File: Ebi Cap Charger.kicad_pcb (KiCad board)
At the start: 2 copper layers, 45 x 100 mm, 31 parts, among them Q1 FET, Q2 FET, U1 LT3751, U2 DA2034-AL, U3 DA2034-AL, U4 DA2034-AL

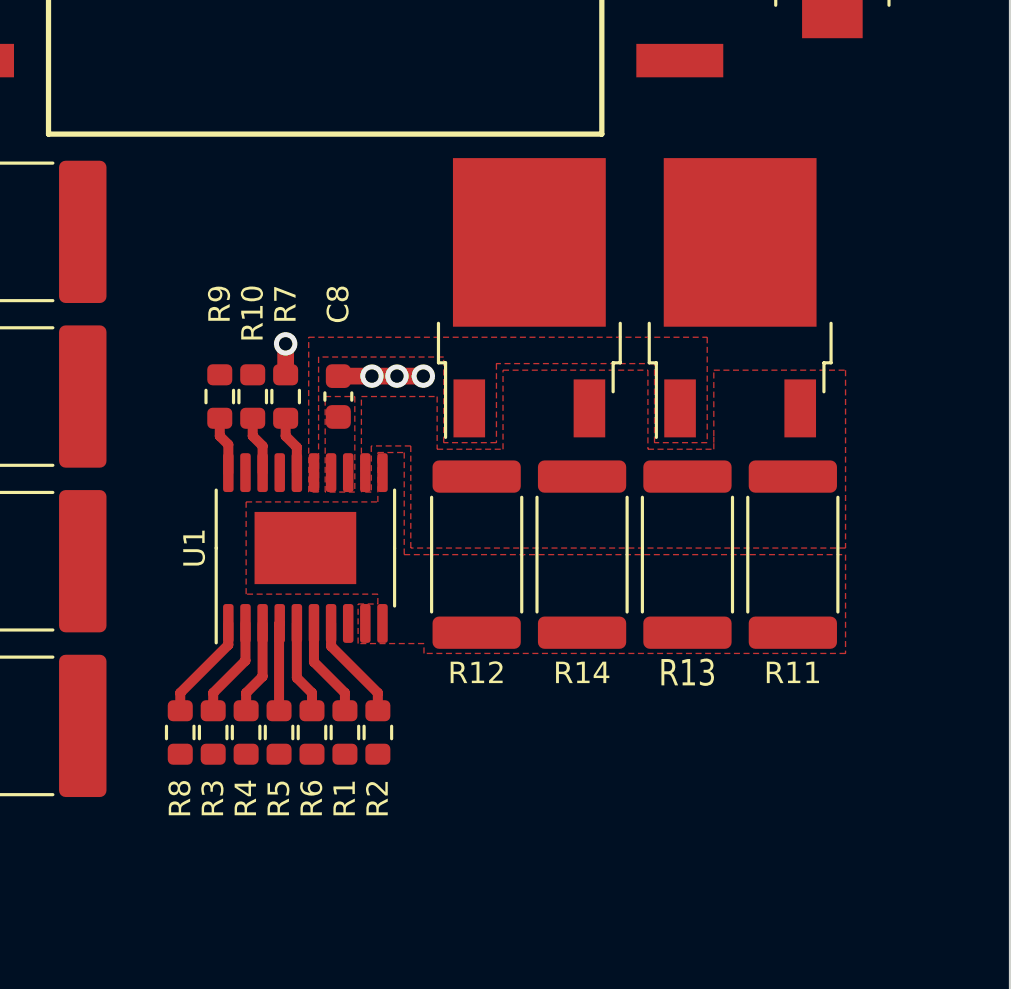
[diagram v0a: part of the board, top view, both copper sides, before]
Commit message: Updated PCB
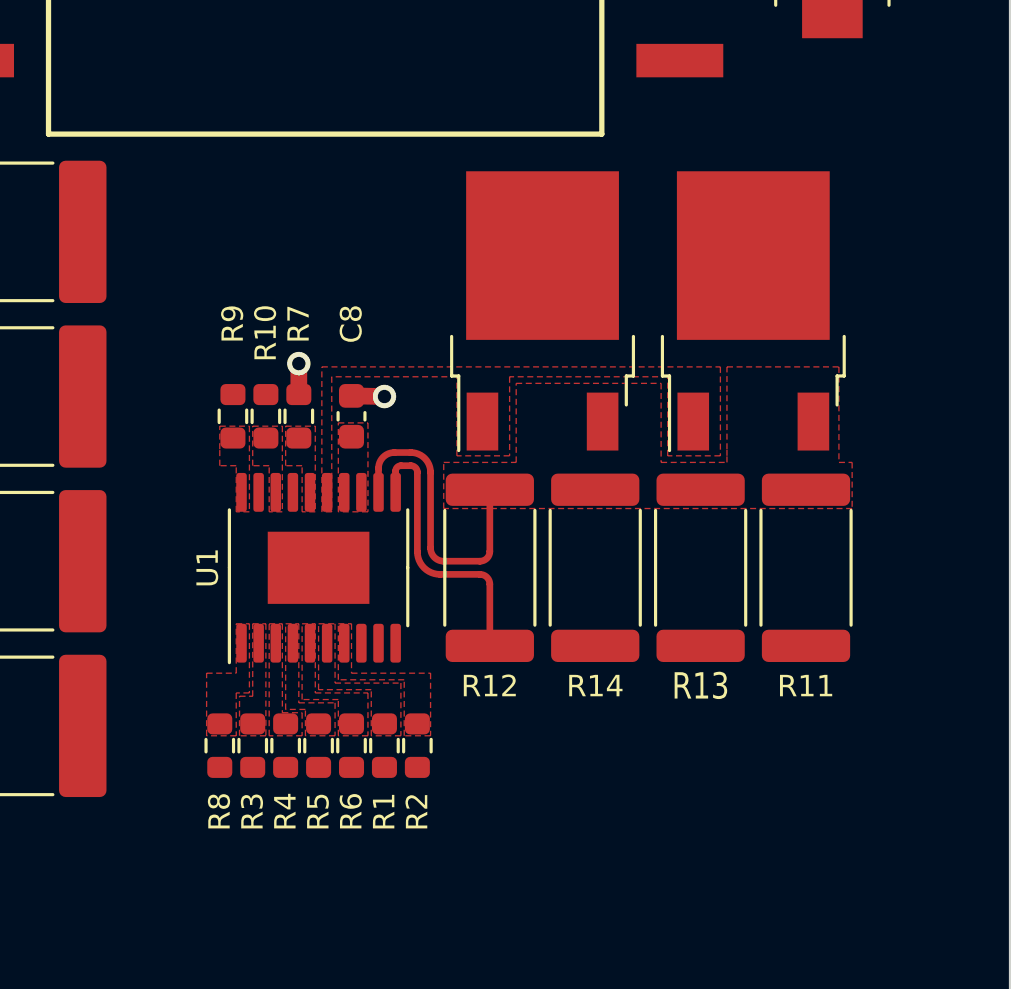
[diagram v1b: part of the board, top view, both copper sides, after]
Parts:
- moved R1 1.58 mm to (168.2, 195.5)
- moved R2 1.58 mm to (169.5, 195.5)
- moved R3 1.58 mm to (163.2, 195.5)
- moved R4 1.58 mm to (164.5, 195.5)
- moved R5 1.58 mm to (165.8, 195.5)
- moved R6 1.58 mm to (167.0, 195.5)
- moved R8 1.58 mm to (162.0, 195.5)
- moved C8 0.90 mm to (167.0, 183.0)
- moved R10 0.90 mm to (163.8, 183.0)
- moved R7 0.90 mm to (165.0, 183.0)
- moved R9 0.90 mm to (162.5, 183.0)
- moved U1 0.90 mm to (165.8, 188.8)
- moved Q1 0.71 mm to (174.2, 179.0)
- moved Q2 0.71 mm to (182.2, 179.0)
- moved R11 0.71 mm to (184.2, 188.8)
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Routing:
- net Net-(Q1-Pad3): track 0.00 -> 11.5 mm
- net GND: track 4.40 -> 13.1 mm, vias 4 -> 2
- net Net-(R8-Pad1): track 4.07 -> 0.00 mm
- net Net-(R2-Pad2): track 4.05 -> 0.00 mm
- net Net-(R3-Pad2): track 3.82 -> 0.00 mm
- net Net-(R1-Pad2): track 3.80 -> 0.00 mm
- net Net-(R4-Pad2): track 3.57 -> 0.00 mm
- net Net-(R6-Pad2): track 3.55 -> 0.00 mm
- net Net-(R5-Pad2): track 3.32 -> 0.00 mm
- net Net-(R7-Pad1): track 2.24 -> 0.00 mm
- net Net-(R10-Pad1): track 2.22 -> 0.00 mm
- net Net-(R9-Pad1): track 2.20 -> 0.00 mm
- added copper zone on F.Cu, net Net-(R1-Pad2)
- added copper zone on F.Cu, net Net-(R10-Pad1)
- added copper zone on F.Cu, net Net-(R2-Pad2)
- added copper zone on F.Cu, net Net-(R3-Pad2)
- added copper zone on F.Cu, net Net-(R4-Pad2)
- added copper zone on F.Cu, net Net-(R5-Pad2)
- added copper zone on F.Cu, net Net-(R6-Pad2)
- added copper zone on F.Cu, net Net-(R7-Pad1)
- added copper zone on F.Cu, net Net-(R8-Pad1)
- added copper zone on F.Cu, net Net-(R9-Pad1)
- removed copper zone on F.Cu, net GND

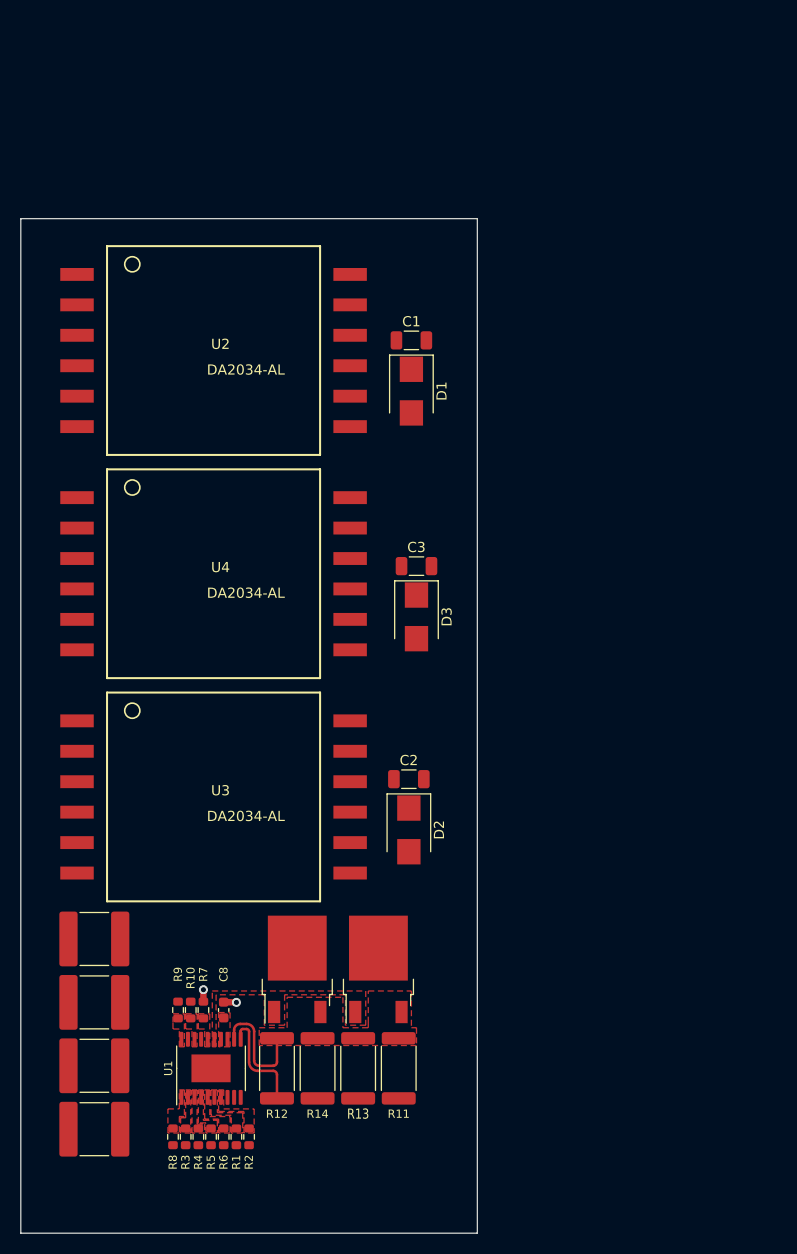
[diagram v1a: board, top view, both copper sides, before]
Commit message: Updated PCB
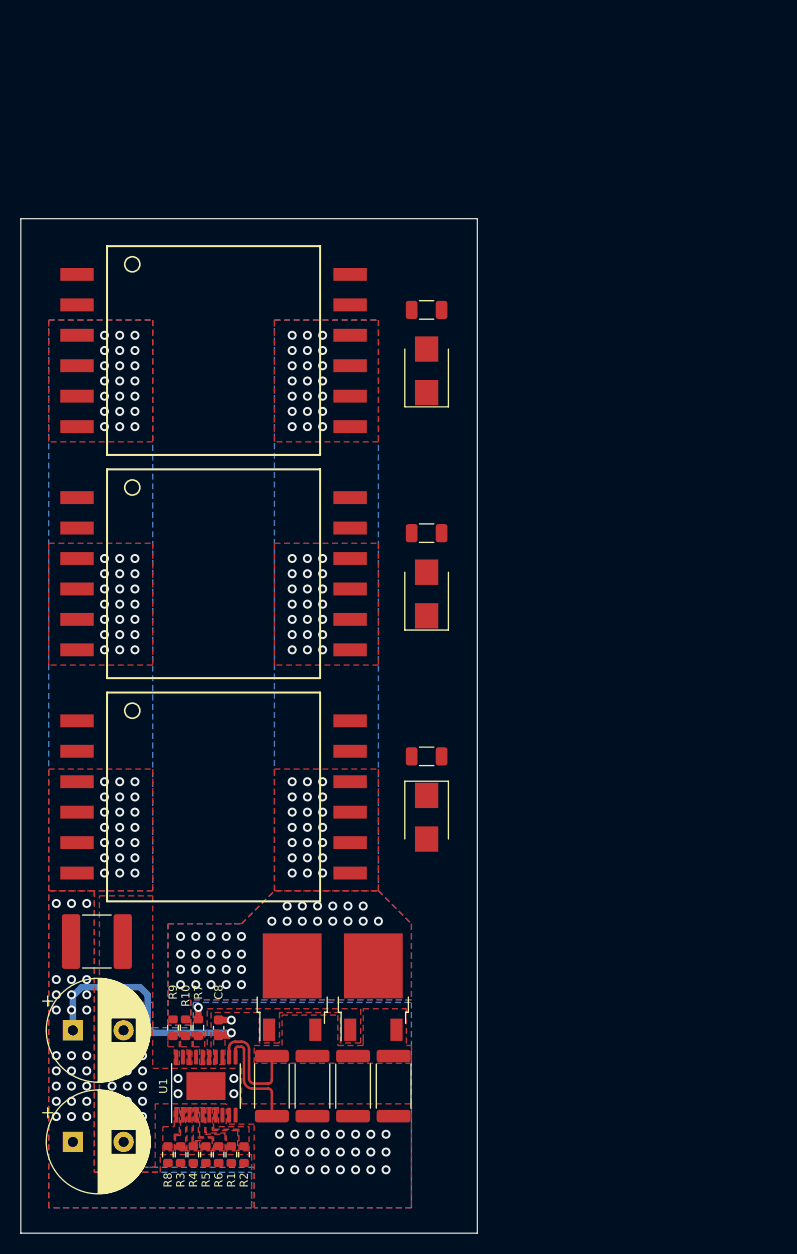
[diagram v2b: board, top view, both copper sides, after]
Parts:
- removed C4: 100uF, Capacitor_SMD:C_2220_5650Metric
- C5, C6: value 100uF -> 470uF; footprint Capacitor_SMD:C_2220_5650Metric -> Capacitor_THT:CP_Radial_D10.0mm_P5.00mm
- moved C7 18.5 mm to (154.5, 176.2)
- moved C6 7.79 mm to (152.1, 196.0)
- moved C5 3.47 mm to (152.1, 185.0)
- moved C3 3.40 mm to (187.0, 136.0), turned to 180 degrees
- moved C1 3.35 mm to (187.0, 114.0), turned to 180 degrees
- moved C2 2.85 mm to (187.0, 158.0), turned to 180 degrees
- moved D1 2.50 mm to (187.0, 120.0), turned to 90 degrees
- moved D3 2.46 mm to (187.0, 142.0), turned to 90 degrees
- moved D2 2.15 mm to (187.0, 164.0)
- moved C8 1.82 mm to (166.5, 184.8)
- moved Q1 1.82 mm to (173.8, 180.8)
- moved Q2 1.82 mm to (181.8, 180.8)
- moved R1 1.82 mm to (167.8, 197.2)
- moved R10 1.82 mm to (163.2, 184.8)
- moved R11 1.82 mm to (183.8, 190.5)
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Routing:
- net Net-(C5-Pad1): track 0.00 -> 24.5 mm, vias 0 -> 91
- net Net-(Q1-Pad2): vias 0 -> 97
- net GND: vias 2 -> 45
- added copper zone on B.Cu, net GND
- added copper zone on F.Cu, net GND
- added copper zone on B.Cu, net Net-(C5-Pad1)
- added copper zone on B.Cu, net Net-(Q1-Pad2)
- added copper zone on F.Cu, net Net-(Q1-Pad2)

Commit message: PCB draft
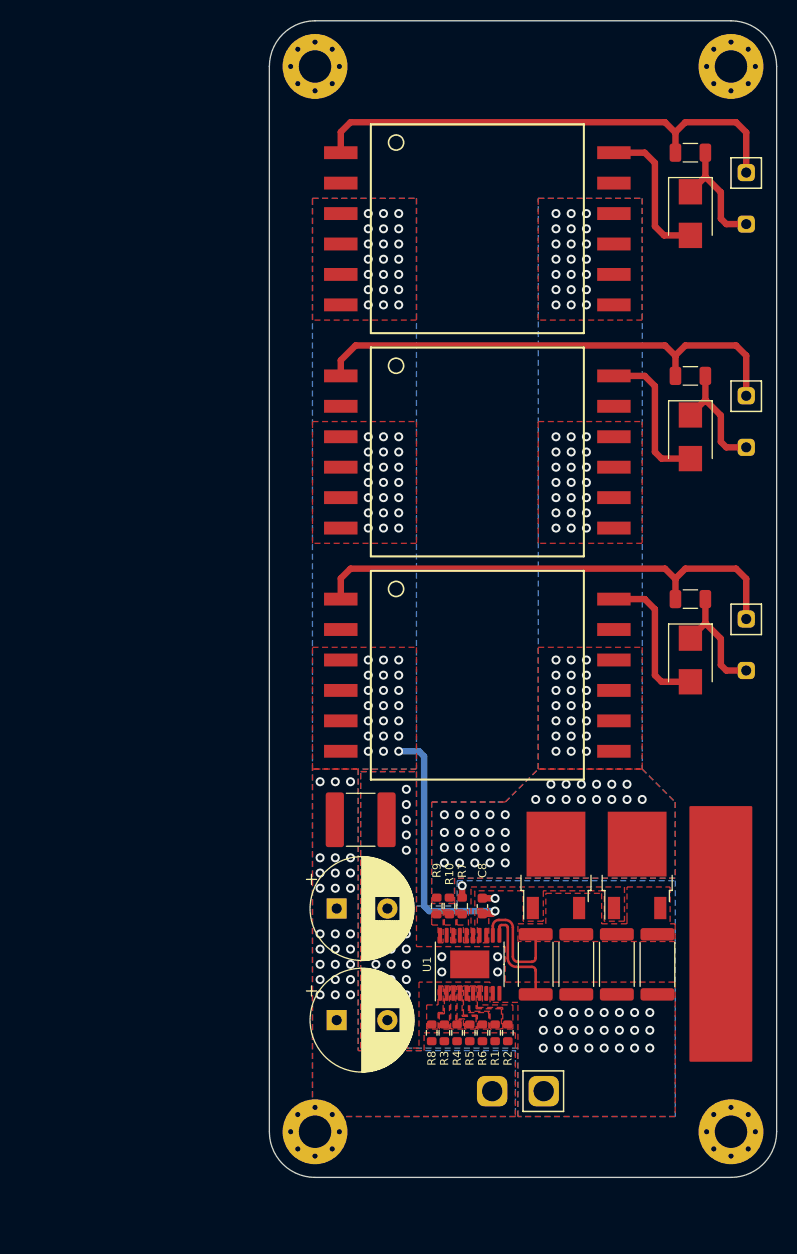
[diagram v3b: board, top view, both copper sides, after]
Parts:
- added G***: LOGO, Art:hvhand3, B.Cu at (192.0, 133.0)
- added H1: MountingHole, MountingHole:MountingHole_3.2mm_M3_Pad_Via, F.Cu at (176.0, 90.0)
- added H2: MountingHole, MountingHole:MountingHole_3.2mm_M3_Pad_Via, F.Cu at (176.0, 195.0)
- added H3: MountingHole, MountingHole:MountingHole_3.2mm_M3_Pad_Via, F.Cu at (217.0, 195.0)
- added H4: MountingHole, MountingHole:MountingHole_3.2mm_M3_Pad_Via, F.Cu at (217.0, 90.0)
- added J1: VIN, Connector_PinHeader_2.54mm:PinHeader_1x02_P2.54mm_Vertical, F.Cu at (193.5, 191.0)
- added J2: C1, Connector_PinHeader_2.54mm:PinHeader_1x02_P2.54mm_Vertical, F.Cu at (218.5, 105.5)
- added J3: C2, Connector_PinHeader_2.54mm:PinHeader_1x02_P2.54mm_Vertical, F.Cu at (218.5, 149.5)
- added J4: C3, Connector_PinHeader_2.54mm:PinHeader_1x02_P2.54mm_Vertical, F.Cu at (218.5, 127.5)
- moved C2 30.3 mm to (213.0, 142.5)
- moved D2 30.3 mm to (213.0, 148.5)
- moved C1 30.3 mm to (213.0, 98.5)
- moved C3 30.3 mm to (213.0, 120.5)
- moved D1 30.3 mm to (213.0, 104.5), turned to -90 degrees
- moved D3 30.3 mm to (213.0, 126.5), turned to -90 degrees
- moved C5 28.6 mm to (178.1, 173.0)
- moved C6 28.6 mm to (178.1, 184.0)
- moved C7 28.6 mm to (180.5, 164.2)
- moved C8 28.6 mm to (192.5, 172.7)
- moved Q1 28.6 mm to (199.8, 168.7)
- moved Q2 28.6 mm to (207.8, 168.7)
- moved R1 28.6 mm to (193.8, 185.2)
- moved R10 28.6 mm to (189.3, 172.7)
- moved R11 28.6 mm to (209.8, 178.5)
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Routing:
- net Net-(C2-Pad2): track 0.00 -> 49.6 mm
- net Net-(C1-Pad2): track 0.00 -> 49.6 mm
- net Net-(C3-Pad2): track 0.00 -> 49.3 mm
- net Net-(D3-Pad2): track 0.00 -> 14.7 mm
- net Net-(D2-Pad2): track 0.00 -> 14.7 mm
- net Net-(D1-Pad2): track 0.00 -> 14.6 mm
- net Net-(C2-Pad1): track 0.00 -> 11.9 mm
- net Net-(C3-Pad1): track 0.00 -> 11.9 mm
- net Net-(C1-Pad1): track 0.00 -> 11.9 mm
- net Net-(C5-Pad1): track 24.5 -> 26.0 mm
- net GND: vias 45 -> 50
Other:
- board size 45 x 100 mm -> 50 x 114 mm
- board text added: "NNNI X EBI 3822 HV CAPACITOR CHARGER"
